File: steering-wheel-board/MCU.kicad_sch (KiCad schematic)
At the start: 15 parts, among them J2 FTSH-107-01-F-DV-K-P-TR, SW1 Y97KT23B5NAFP, U5 STM32G441KBTx, Y1 ECS-240-8-37B-CKY-TR

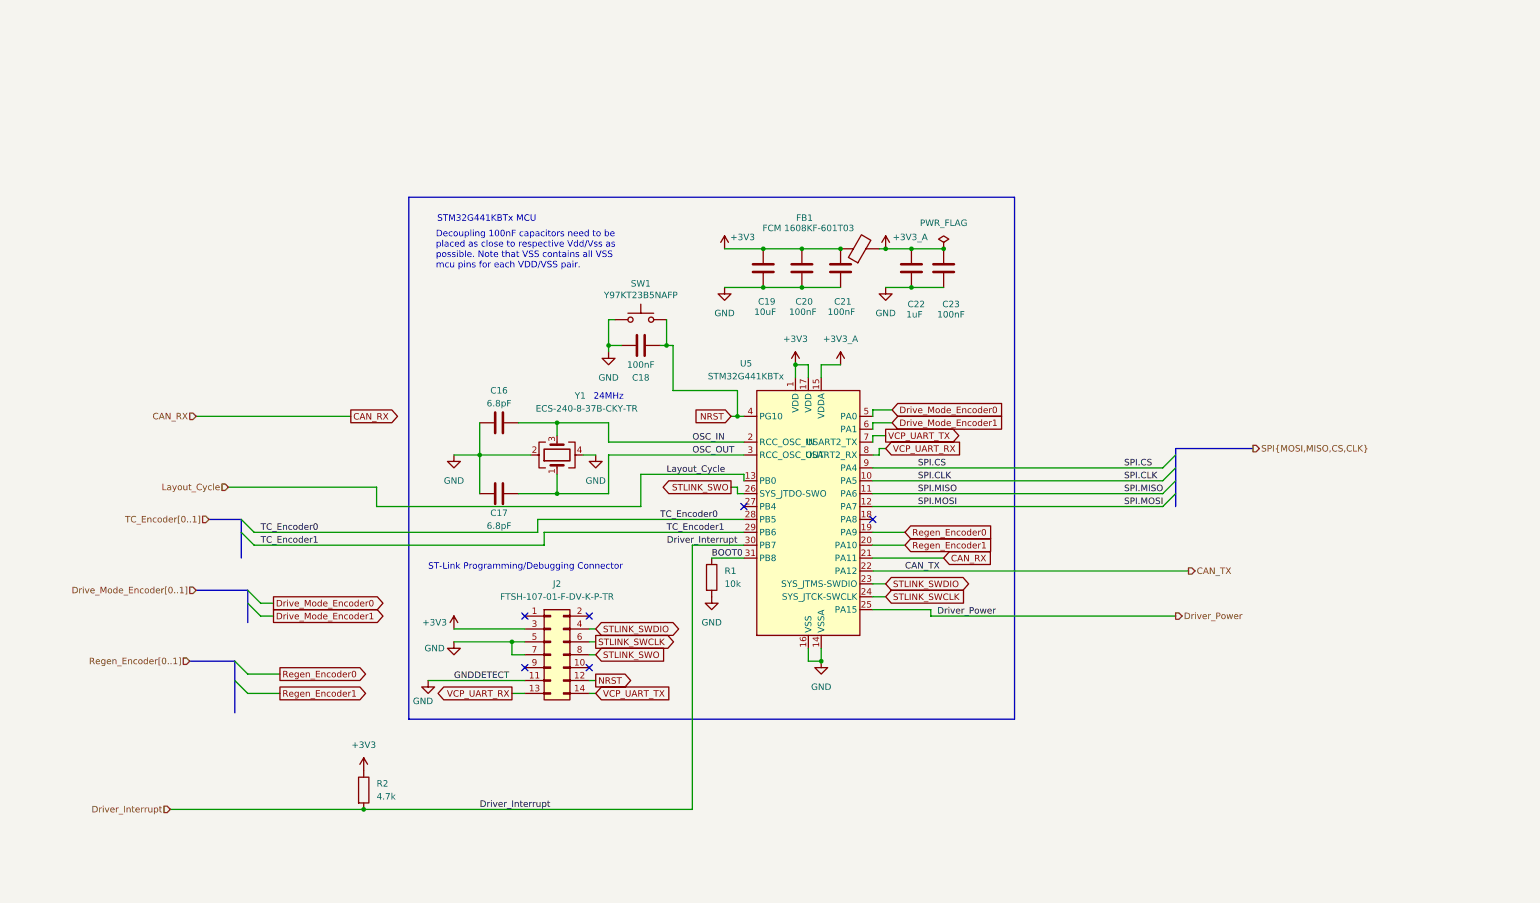
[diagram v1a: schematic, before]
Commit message: revised steering wheel board schematic to address PR comments; replaced encoders with resistor ladders for dials, and added dials into schematic
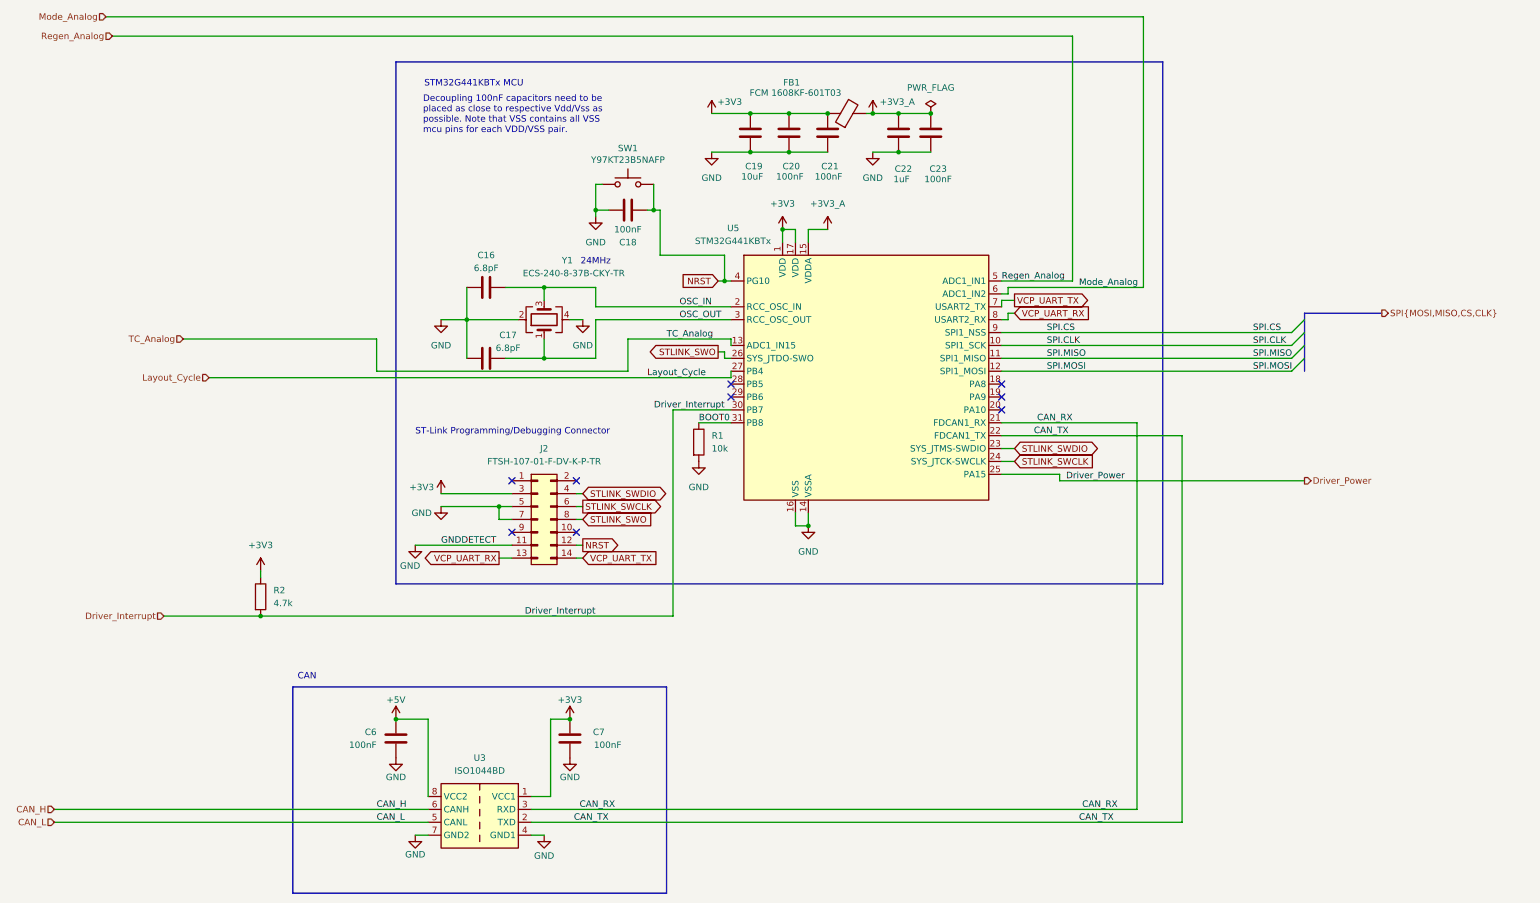
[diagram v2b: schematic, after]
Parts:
- added C6, C7: 100nF, Capacitor_SMD:C_0805_2012Metric_Pad1.18x1.45mm_HandSolder, symbol Device:C
- added U3: ISO1044BD, Package_SO:SOIC-8_3.9x4.9mm_P1.27mm, symbol Interface_CAN_LIN:ISO1044BD
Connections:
- net +3V3: now also C7.1, U3.1 (VCC1)
- net CAN_RX: now also U3.3 (RXD)
- net CAN_TX: now also U3.2 (TXD)
- net GND: now also C6.2, C7.2, U3.4 (GND1), U3.7 (GND2)
- net Layout_Cycle: now also U5.27 (PB4); no longer U5.13 (PB0)
- net Drive_Mode_Encoder0 renamed Regen_Analog
- net Drive_Mode_Encoder1 renamed Mode_Analog
- net Regen_Encoder0: no longer names the net of U5.19 (PA9)
- net Regen_Encoder1: no longer names the net of U5.20 (PA10)
- net TC_Encoder0: no longer names the net of U5.28 (PB5)
- net TC_Encoder1: no longer names the net of U5.29 (PB6)
- new net +5V: C6.1, U3.8 (VCC2)
- new net CAN_H: U3.6 (CANH)
- new net CAN_L: U3.5 (CANL)
- new net TC_Analog: U5.13 (PB0)
- no-connect marks 6 -> 9
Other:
- note added: "CAN"
- moved on the sheet: C16, C17, C18, C19, C20, C21, C22, C23, FB1, J2, R1, R2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
